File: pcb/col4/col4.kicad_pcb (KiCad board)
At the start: 2 copper layers, 81.8 x 17.6 mm, 12 parts

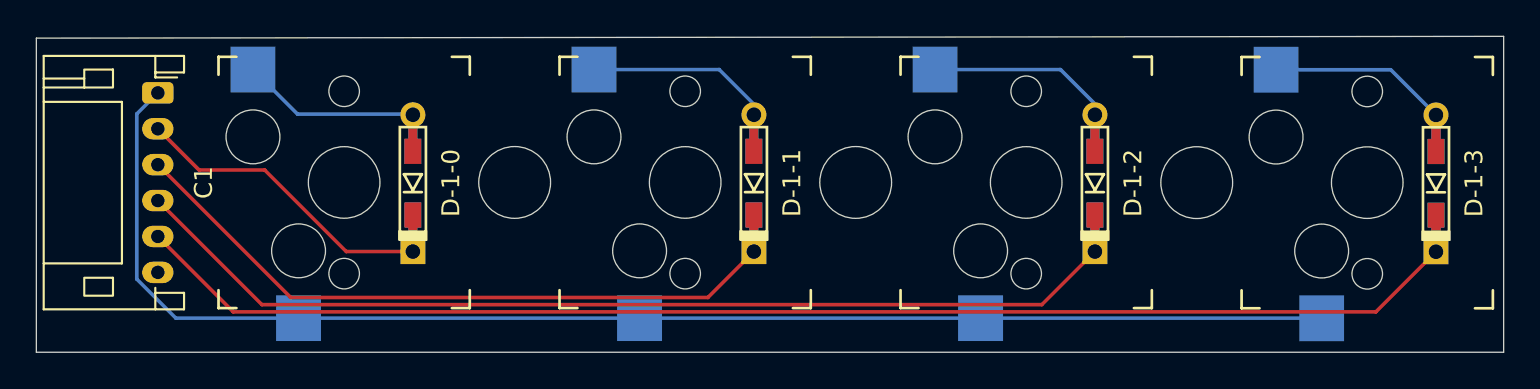
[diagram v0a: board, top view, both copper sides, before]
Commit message: adjusted  col unit pcb
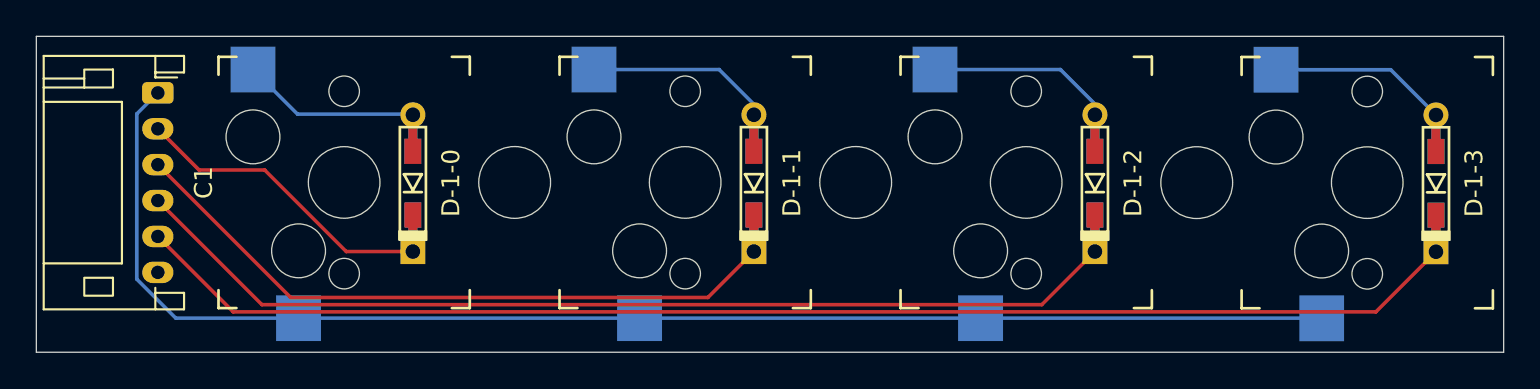
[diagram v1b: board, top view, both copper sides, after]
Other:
- outline, holes or cut-outs redrawn
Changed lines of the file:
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@@
 	)
 	(gr_line
-		(start 34.4 41.1)
+		(start 34.4 41)
 		(end 34.4 58.599958)
 		(stroke
@@
 	(gr_line
 		(start 116.15 41)
-		(end 34.4 41.1)
+		(end 34.4 41)
 		(stroke
 			(width 0.05)
@@
 	(gr_line
 		(start 116.15 58.6)
-		(end 34.4 58.599945)
+		(end 34.4 58.6)
 		(stroke
 			(width 0.05)
@@
 	)
 	(segment
+		(start 103.47 42.86)
+		(end 109.86 42.86)
+		(width 0.2)
+		(layer "B.Cu")
+		(net "Net-(D-1-3-A)")
+	)
+	(segment
+		(start 109.86 42.86)
+		(end 112.38 45.38)
+		(width 0.2)
+		(layer "B.Cu")
+		(net "Net-(D-1-3-A)")
+	)
+	(segment
 		(start 93.379005 44.77)
 		(end 93.379005 45.37)
@@
 		(net "Net-(D-1-2-A)")
 	)
-	(segment
-		(start 103.47 42.86)
-		(end 109.86 42.86)
-		(width 0.2)
-		(layer "B.Cu")
-		(net "Net-(D-1-3-A)")
-	)
-	(segment
-		(start 109.86 42.86)
-		(end 112.38 45.38)
-		(width 0.2)
-		(layer "B.Cu")
-		(net "Net-(D-1-3-A)")
-	)
 	(embedded_fonts no)
